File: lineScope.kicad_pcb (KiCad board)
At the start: 2 copper layers, 100 x 50 mm, 86 parts, among them J1 Conn_01x02, J2 Conn_01x02, J3 Conn_01x03, J4 Conn_01x03, J5 Conn_01x03, J7 Conn_Coaxial, J8 Conn_Coaxial, J9 Conn_01x04, K1 HE721A0500, K2 HE721A0500, Q1 BC847, Q2 BC847, U1 ADuM3190, U2 ADuM3190, U3 L78L09_SOT89, U4 LM4040DBZ-2.0, U5 L78L09_SOT89, U6 LM358

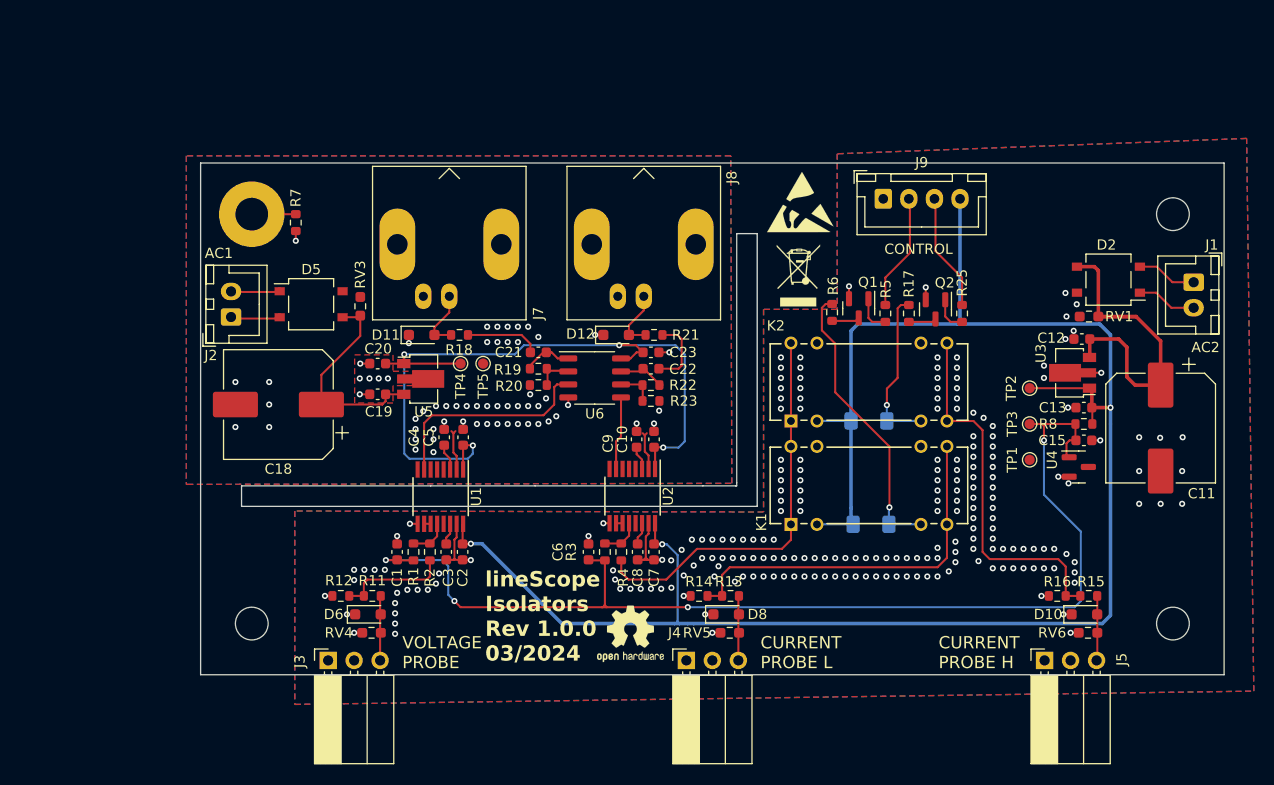
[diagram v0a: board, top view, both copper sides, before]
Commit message: Redesign pcb
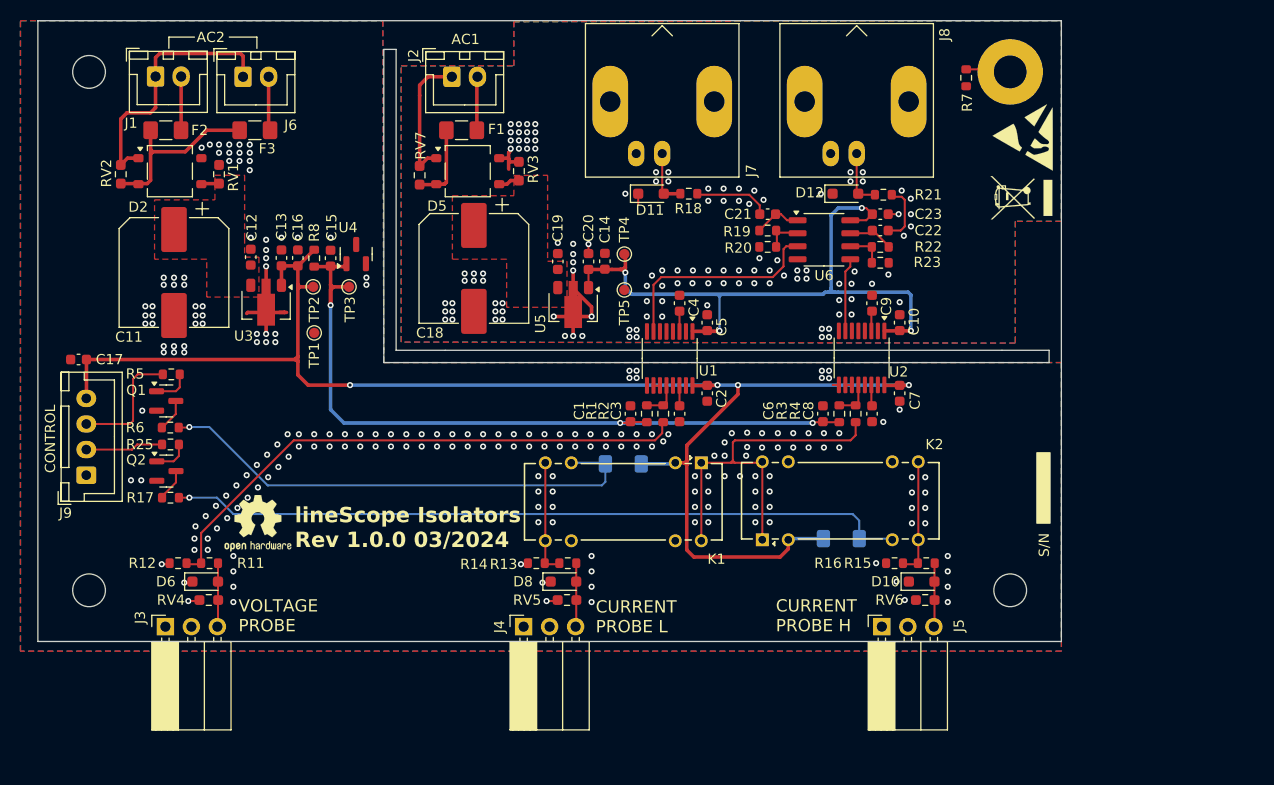
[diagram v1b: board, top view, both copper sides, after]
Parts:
- added C14: 1u, Capacitor_SMD:C_0603_1608Metric, F.Cu at (139.5, 59.6)
- added C16: 1u, Capacitor_SMD:C_0603_1608Metric, F.Cu at (109.5, 59.3)
- added C17: 100n, Capacitor_SMD:C_0603_1608Metric, F.Cu at (88.1, 69.2)
- added F1: 160mA, Fuse:Fuse_1206_3216Metric_Pad1.42x1.75mm_HandSolder, F.Cu at (125.5, 46.8)
- added F2: 160mA, Fuse:Fuse_1206_3216Metric_Pad1.42x1.75mm_HandSolder, F.Cu at (96.6, 46.8)
- added F3: 160mA, Fuse:Fuse_1206_3216Metric_Pad1.42x1.75mm_HandSolder, F.Cu at (105.3, 46.8)
- added J6: Conn_01x02, Connector_JST:JST_XH_B2B-XH-A_1x02_P2.50mm_Vertical, F.Cu at (104.2, 41.6)
- added RV2: MCVZ0603M180AGT, Resistor_SMD:R_0603_1608Metric_Pad0.98x0.95mm_HandSolder, F.Cu at (92.2, 51.1)
- added RV7: MCVZ0603M180AGT, Resistor_SMD:R_0603_1608Metric_Pad0.98x0.95mm_HandSolder, F.Cu at (121.4, 51.2)
- moved H6 106.8 mm to (89.1, 41.1)
- moved J1 103.4 mm to (95.6, 41.5), turned to 0 degrees
- moved C11 97.6 mm to (97.4, 60.7)
- moved D2 92.3 mm to (97.0, 50.8), turned to 0 degrees
- moved RV1 86.1 mm to (101.8, 51.1), turned to 90 degrees
- moved J9 82.4 mm to (88.8, 80.5), turned to 90 degrees
- moved C12 81.6 mm to (104.9, 59.2), turned to 90 degrees
- moved C13 79.8 mm to (107.9, 59.3), turned to 90 degrees
- moved U3 78.8 mm to (106.4, 63.9), turned to -90 degrees
- moved R25 78.4 mm to (97.1, 77.5), turned to 180 degrees
- moved R8 76.9 mm to (111.1, 59.3), turned to -90 degrees
- moved Q2 76.8 mm to (96.7, 80.1), turned to 0 degrees
- moved C15 75.7 mm to (112.7, 59.3), turned to 90 degrees
- moved H1 75.4 mm to (179.1, 41.1)
- moved R17 74.4 mm to (97.1, 82.7), turned to 180 degrees
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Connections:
- D2 pad 1: Net-(J1-Pin_2) -> Net-(J1-Pin_1)
- D2 pad 2: Net-(J1-Pin_1) -> Net-(D2-Pad2)
- D5 pad 1: Net-(J2-Pin_2) -> Net-(J2-Pin_1)
- D5 pad 2: Net-(J2-Pin_1) -> Net-(D5-Pad2)
- J9 pad 2: /Modules Connector/Probe_L -> /Modules Connector/Probe_H
- J9 pad 3: /Modules Connector/Probe_H -> /Modules Connector/Probe_L
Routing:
- net Net-(D9-A): track 16.0 -> 72.4 mm
- net VCC2: track 192.6 -> 146.3 mm, vias 3 -> 4
- net /Isolators/IN.V: track 11.0 -> 54.8 mm
- net Net-(D2-+): track 42.0 -> 1.75 mm
- net VREF2: track 109.4 -> 74.2 mm, vias 4 -> 3
- net Net-(K1-Pad7): track 37.0 -> 11.4 mm
- net Net-(K2-Pad7): track 36.4 -> 11.5 mm
- net Net-(D7-A): track 28.2 -> 49.3 mm
- net Net-(J1-Pin_1): track 5.88 -> 26.1 mm
- net Net-(D5-+): track 20.9 -> 2.07 mm
- net Net-(D2-Pad2): track 0.00 -> 17.9 mm
- net GND2: track 28.6 -> 18.1 mm, vias 218 -> 213
- net Net-(D5-Pad2): track 0.00 -> 7.99 mm
- net Net-(J2-Pin_1): track 5.16 -> 12.8 mm
- net Net-(J6-Pin_2): track 0.00 -> 5.28 mm
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- added copper zone on F.Cu, net Net-(D2-+)
- added copper zone on F.Cu, net Net-(D5-+)
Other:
- board size 100 x 50 mm -> 100 x 60.6 mm
- board text added: "S/N"
